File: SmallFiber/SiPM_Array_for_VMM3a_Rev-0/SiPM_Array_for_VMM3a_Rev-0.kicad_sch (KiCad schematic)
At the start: 21 parts, among them J1 ERM6-30-01.5-L-DV-A-K-TR, J2 ERM6-30-01.5-L-DV-A-K-TR

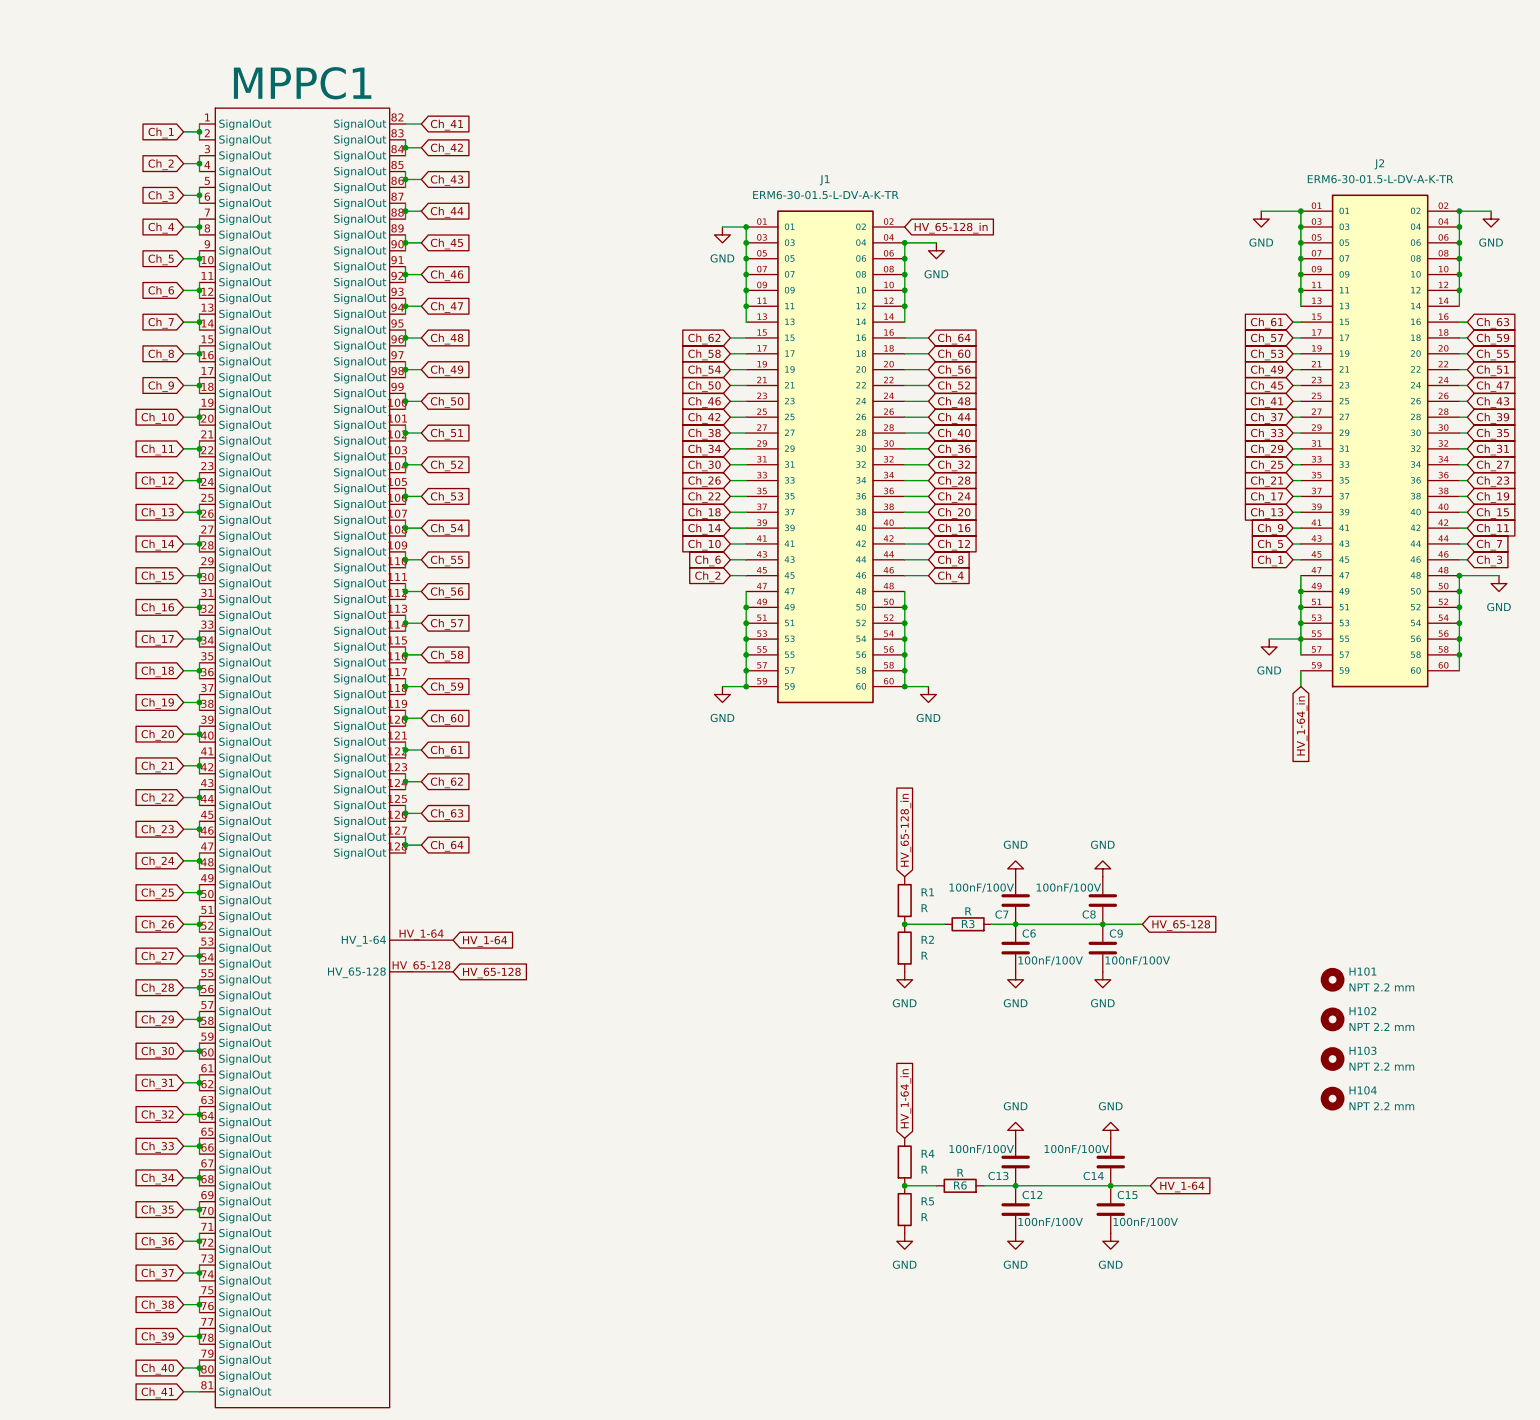
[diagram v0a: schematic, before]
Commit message: g
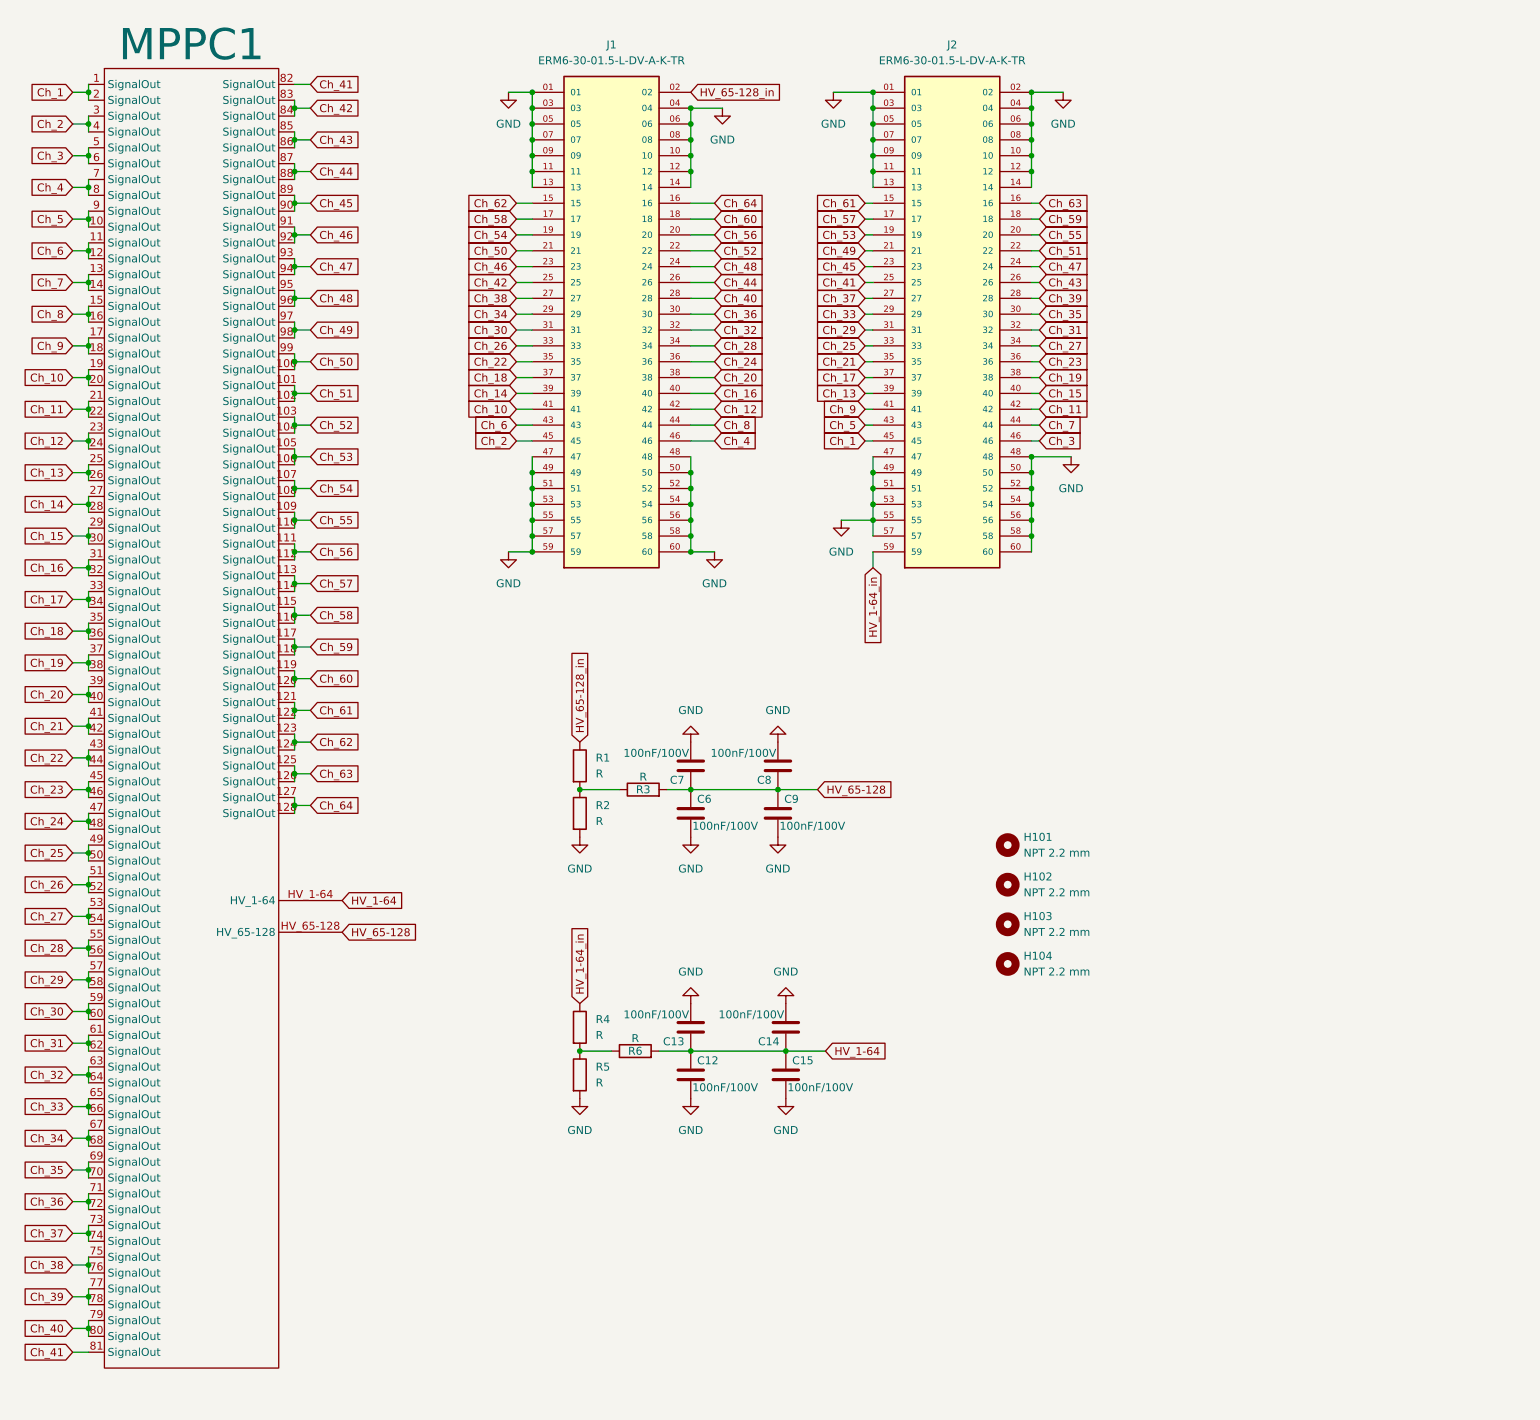
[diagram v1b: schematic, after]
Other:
- title: (none) -> Hamamatsu S13552 carrier board
- moved on the sheet: C12, C13, C14, C15, C6, C7, C8, C9, H101, H102, H103, H104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
